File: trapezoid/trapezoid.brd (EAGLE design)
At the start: 90 x 35 mm, 30 parts, among them IC2 LGD20H, U1 MMA8452Q, U2 microSD, U4 MCP73831, Y1 CRYSTAL.ABS25

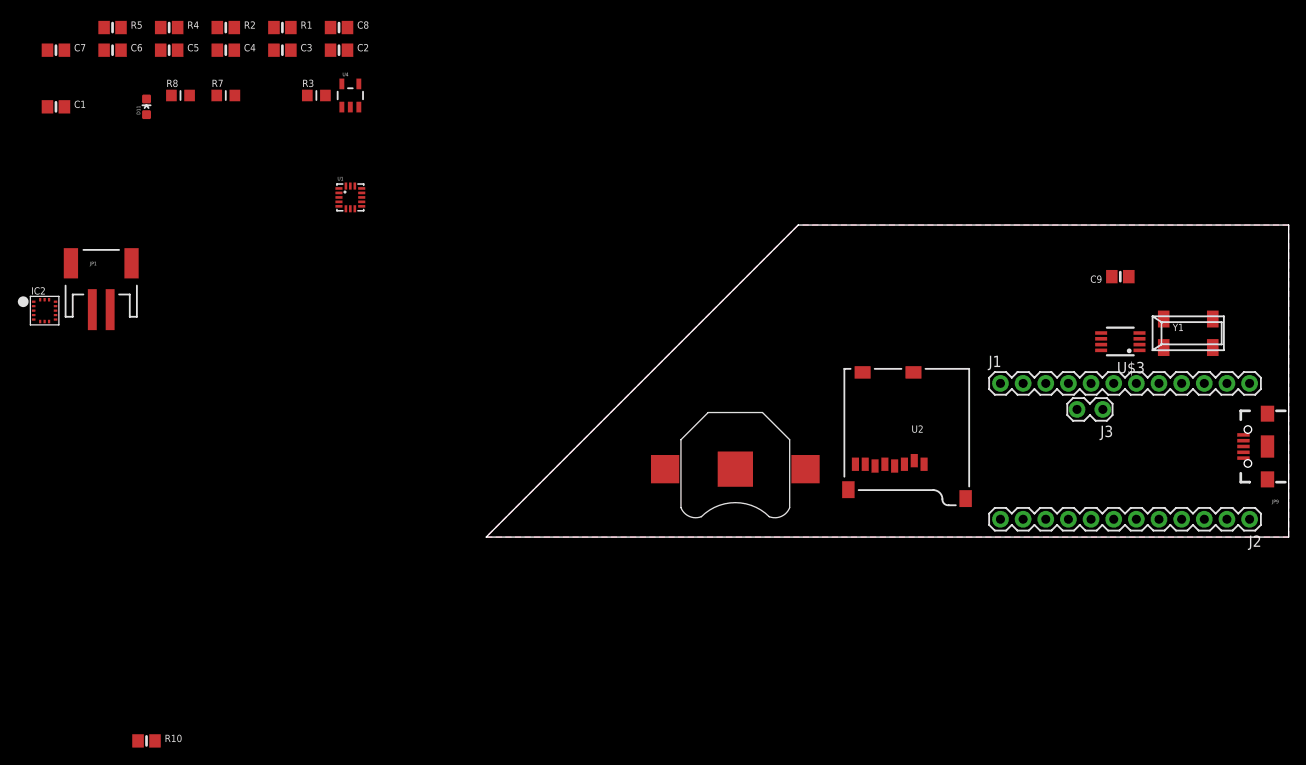
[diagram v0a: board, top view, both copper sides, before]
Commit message: placed rtc and usd
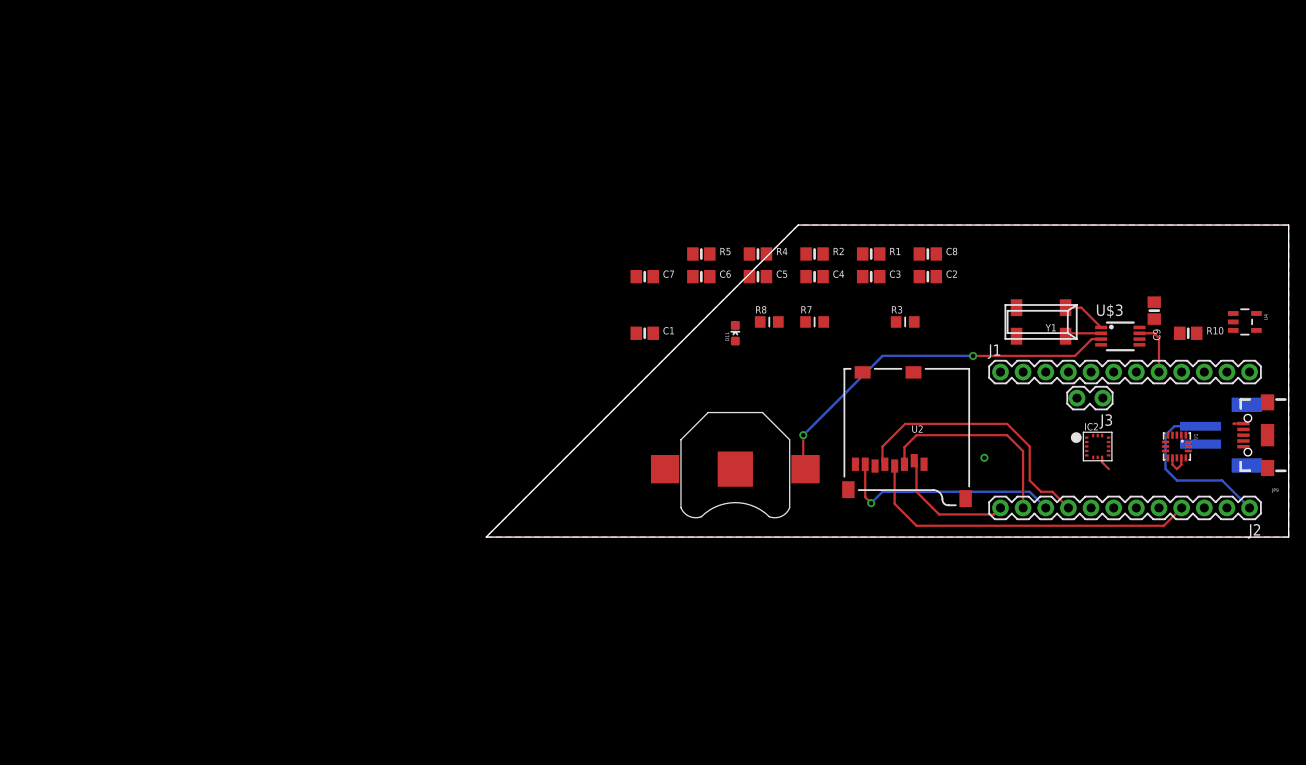
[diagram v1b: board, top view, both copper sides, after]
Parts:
- moved JP1 128.2 mm to (83.8, 11.4), flipped to the bottom, turned to 90 degrees
- moved R10 125.5 mm to (78.7, 22.9)
- moved IC2 119.1 mm to (68.6, 10.2)
- moved U4 103.5 mm to (85.1, 24.1), turned to 270 degrees
- moved U1 96.8 mm to (77.5, 10.2), turned to 270 degrees
- moved C2 70.8 mm to (49.5, 29.2)
- moved C5 70.8 mm to (30.5, 29.2)
- moved C8 70.8 mm to (49.5, 31.8)
- moved D11 70.8 mm to (27.9, 22.9)
- moved R3 70.8 mm to (47.0, 24.1)
- moved R4 70.8 mm to (30.5, 31.8)
- moved C1 70.8 mm to (17.8, 22.9)
- moved C3 70.8 mm to (43.2, 29.2)
- moved C4 70.8 mm to (36.8, 29.2)
- moved C6 70.8 mm to (24.1, 29.2)
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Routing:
- net N$4: track 0.00 -> 41.8 mm, vias 0 -> 2
- net +3V3: track 0.00 -> 38.3 mm
- net SCK: track 0.00 -> 30.1 mm
- net MISO: track 0.00 -> 25.5 mm, vias 0 -> 1
- net MOSI: track 0.00 -> 22.9 mm
- net V_RAW: track 0.00 -> 19.4 mm
- net SD_CS: track 0.20 -> 14.6 mm
- net SQW/INT: track 0.00 -> 6.23 mm
- net GND: track 0.00 -> 5.70 mm, vias 0 -> 1
- net N$5: track 0.00 -> 4.91 mm
- net N$2: track 0.00 -> 4.13 mm
